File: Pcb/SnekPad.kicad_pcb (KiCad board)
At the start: 2 copper layers, 90.5 x 64.3 mm, 16 parts, among them J1 OLED_128x64, SW1 RotaryEncoder_Switch, U1 Raspberry_Pi_Pico

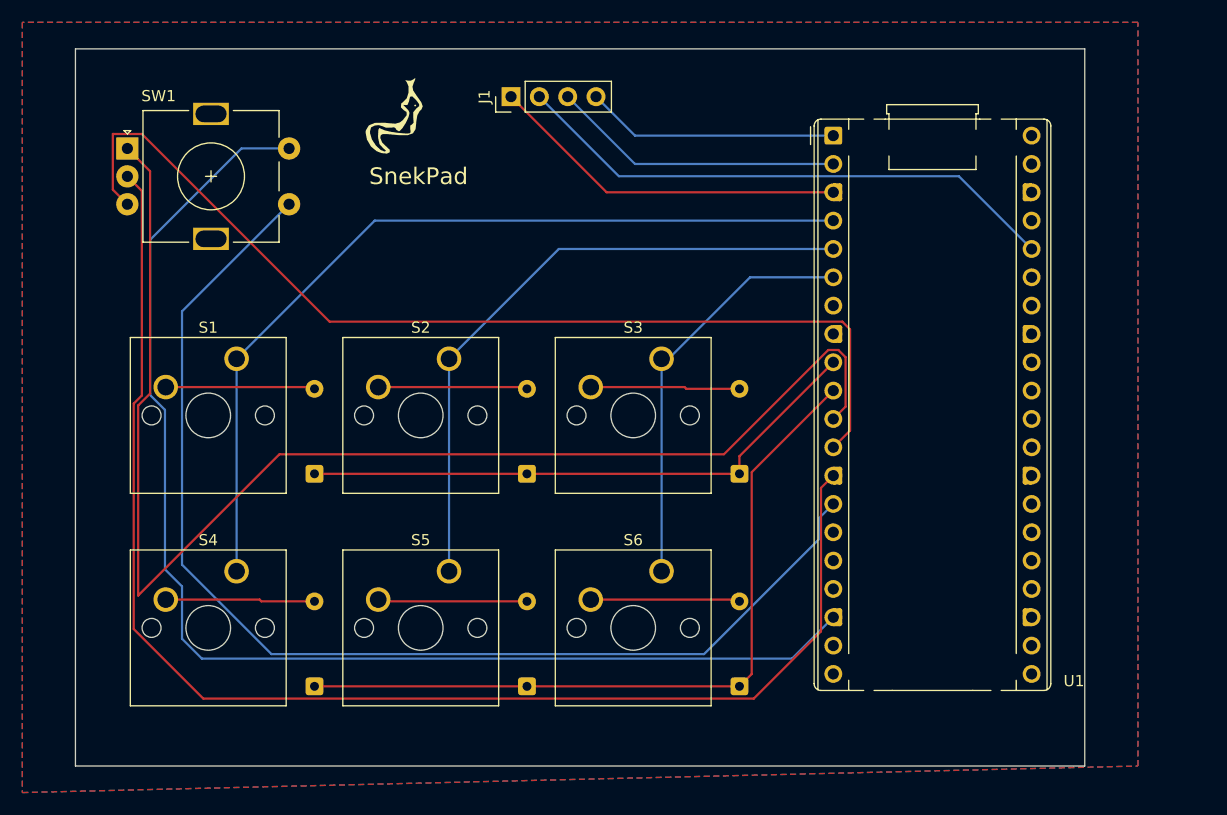
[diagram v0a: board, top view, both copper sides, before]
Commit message: Update SnekPad.kicad_pcb
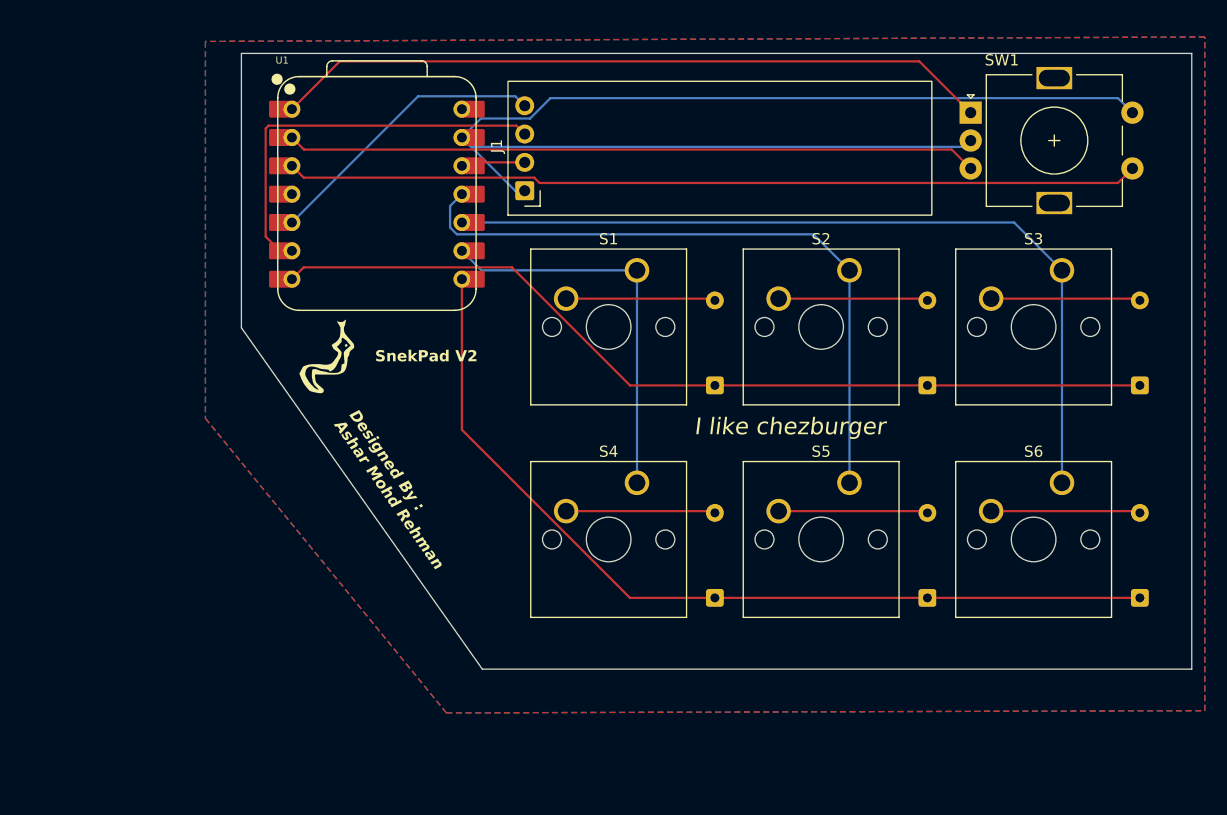
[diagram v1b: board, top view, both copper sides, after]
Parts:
- removed SnekPad: LOGO, snek.preety:snek
- added G***: LOGO, snek.preety:snek1, F.Cu at (127.4, 99.8)
- J1: value OLED_128x64 -> OLED_128x32; footprint Connector_PinHeader_2.54mm:PinHeader_1x04_P2.54mm_Vertical -> Hackclub Footprints:OLED_0.91_128x32
- U1: value Raspberry_Pi_Pico -> XIAO-RP2040-DIP; footprint Module:RaspberryPi_Pico_Common_THT -> OPL Library:XIAO-RP2040-DIP
- moved SW1 75.7 mm to (185.0, 77.2)
- moved U1 41.3 mm to (131.8, 84.5)
- moved D2 36.8 mm to (181.2, 101.6)
- moved D3 36.8 mm to (200.2, 101.6)
- moved D5 36.8 mm to (181.2, 120.7)
- moved D6 36.8 mm to (200.2, 120.7)
- moved S1 36.8 mm to (155.1, 91.3)
- moved S3 36.8 mm to (193.2, 91.3)
- moved S4 36.8 mm to (155.1, 110.3)
- moved S6 36.8 mm to (193.2, 110.3)
- moved D1 36.8 mm to (162.1, 101.6)
- moved D4 36.8 mm to (162.1, 120.7)
- moved S2 36.8 mm to (174.2, 91.3)
- moved S5 36.8 mm to (174.2, 110.3)
- moved J1 8.52 mm to (145.1, 84.2)
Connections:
- J1 pad 1: /GND -> GND
- SW1 pad C: /Enc C -> GND
- SW1 pad S2: /Enc SW2 -> GND
- U1 pad 1: /SDA -> /Enc A
- U1 pad 10: /Row 2 -> /Col 3
- U1 pad 11: /Enc A -> /Col 2
- U1 pad 12: /Enc B -> /VCC
- U1 pad 13: /Enc C -> GND
- U1 pad 14: /Enc SW1 -> unconnected-(U1-VBUS-Pad14)
- U1 pad 2: /SCL -> /Enc B
- U1 pad 3: /GND -> /Enc SW1
- U1 pad 4: /Col 1 -> unconnected-(U1-GPIO29/ADC3/A3-Pad4)
- U1 pad 5: /Col 2 -> /SDA
- U1 pad 6: /Col 3 -> /SCL
- U1 pad 7: unconnected-(U1-GPIO5-Pad7) -> /Row 1
- U1 pad 8: unconnected-(U1-GND-Pad8) -> /Row 2
- U1 pad 9: /Row 1 -> /Col 1
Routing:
- net /Enc C: track 122.5 -> 0.00 mm
- net GND: track 0.00 -> 115.9 mm
- net /Enc SW2: track 113.5 -> 0.00 mm
- net /Enc A: track 120.2 -> 64.5 mm
- net /VCC: track 49.8 -> 5.76 mm
- net /Col 1: track 77.7 -> 35.5 mm
- net /Col 3: track 37.5 -> 74.6 mm
- net /GND: track 32.4 -> 0.00 mm
- net /Enc B: track 91.4 -> 62.0 mm
- net /Row 1: track 51.6 -> 80.8 mm
- net /Enc SW1: track 104.7 -> 76.5 mm
- net /Row 2: track 68.1 -> 80.5 mm
- net /SCL: track 26.3 -> 36.2 mm
- net /SDA: track 22.7 -> 25.9 mm
- net /Col 2: track 57.6 -> 59.9 mm
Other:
- board size 90.5 x 64.3 mm -> 85.2 x 55.2 mm
- board text added: "Designed By : Ashar Mohd Rehman"
- board text added: "I like chezburger"
- board text added: "SnekPad V2"
- board text removed: "${REFERENCE}"
